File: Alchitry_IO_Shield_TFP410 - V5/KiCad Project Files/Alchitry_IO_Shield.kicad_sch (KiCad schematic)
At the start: 1 part, among them U1 boardmezzanine_new

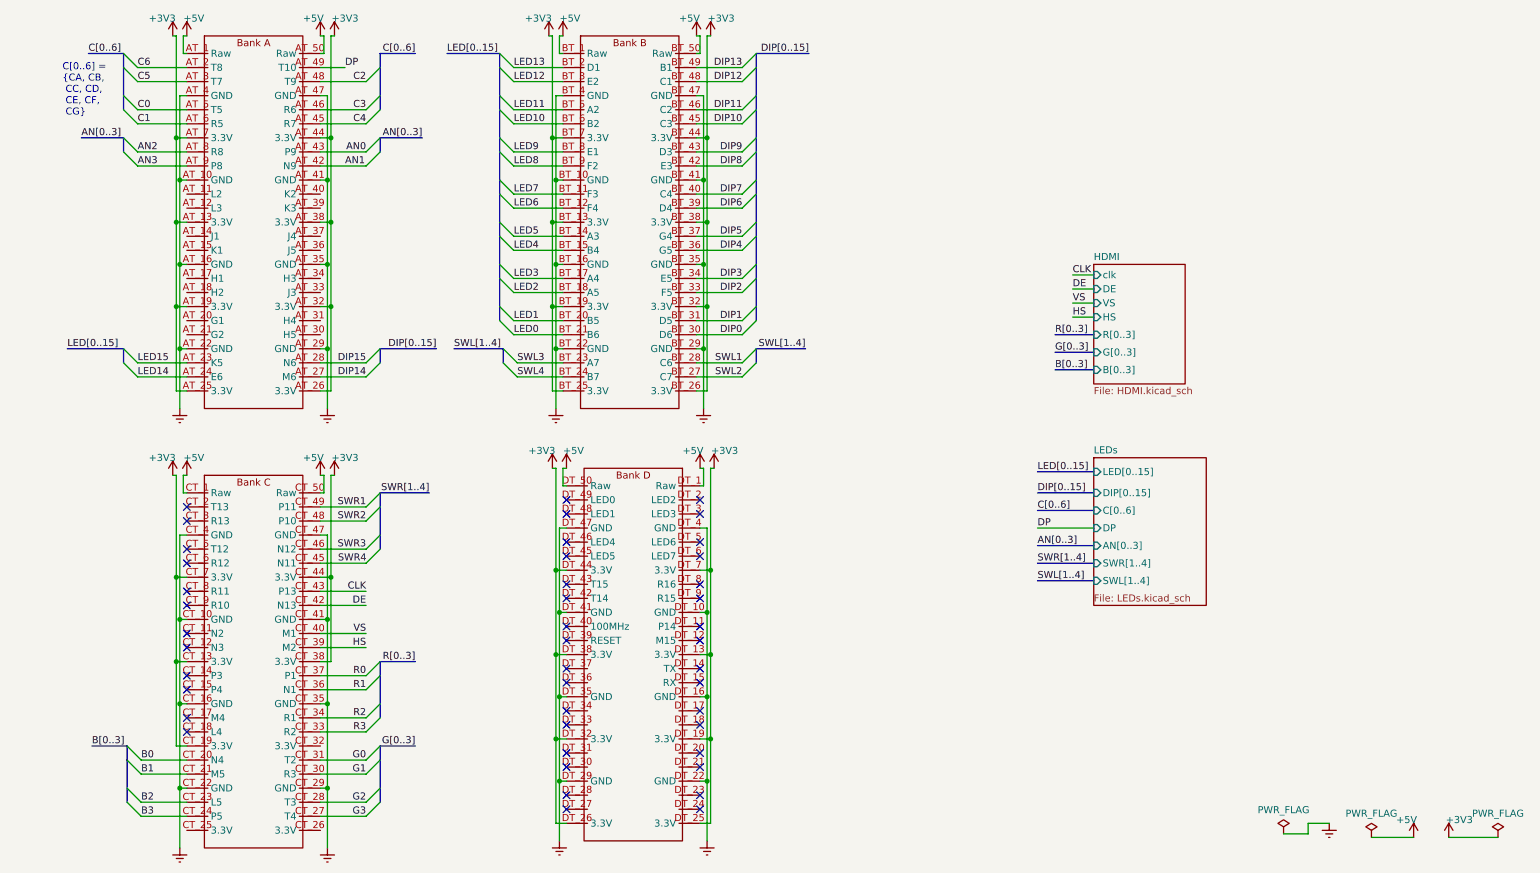
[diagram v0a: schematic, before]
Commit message: started new shield
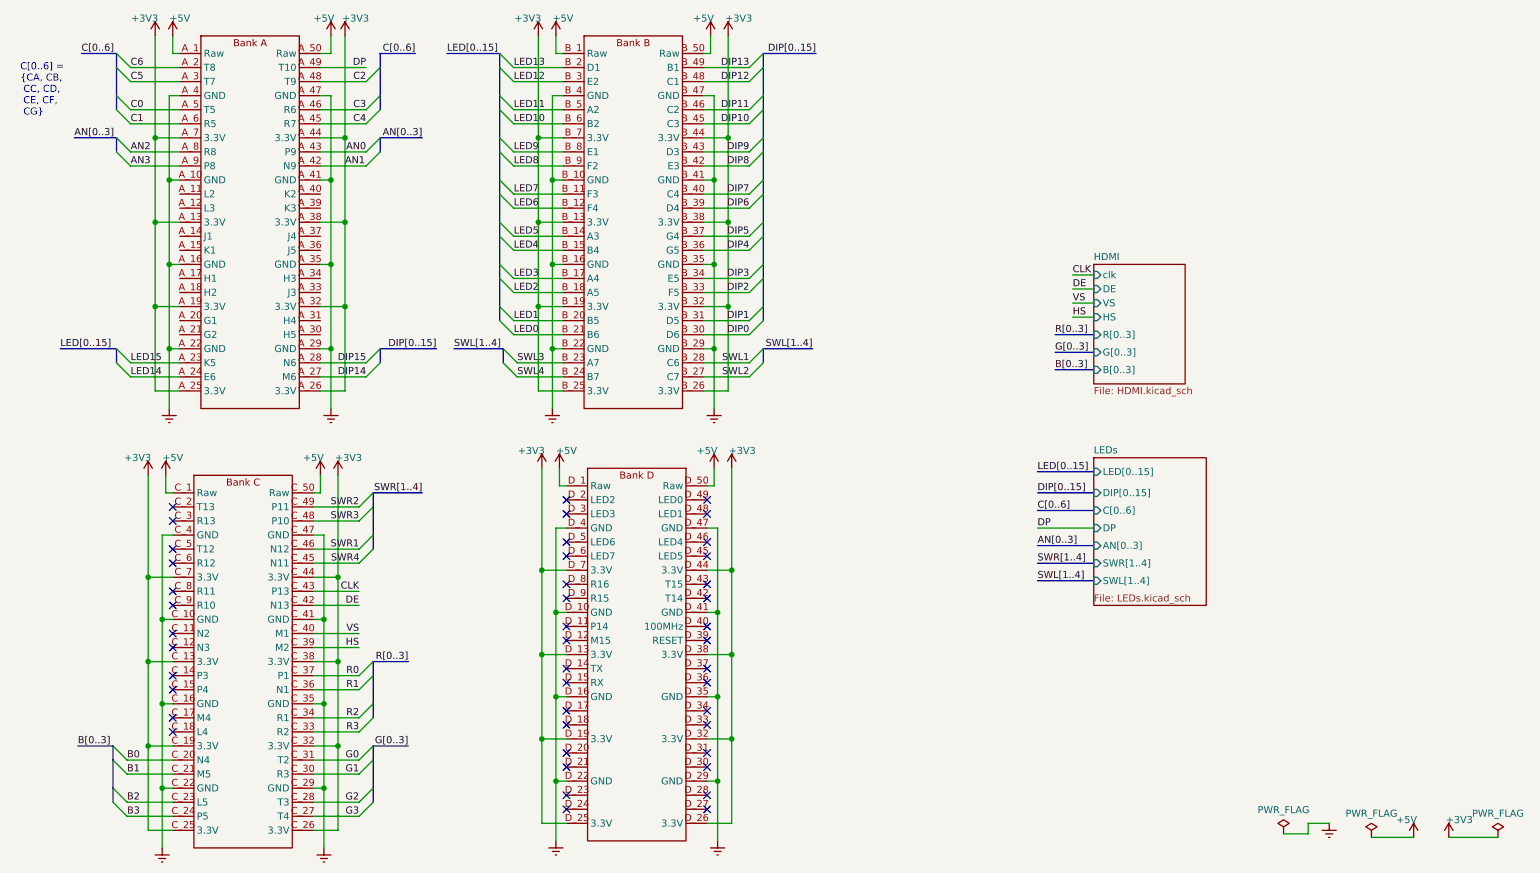
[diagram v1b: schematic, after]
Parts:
- removed U1: boardmezzanine_new, Custom_Parts:Alchitry_Top_Bottom, symbol Custom_Symbols:Adaptor_both-alchitry_symbols
- added U1: Alchitry_Single, Alchitry_Footprints:Alchitry_Bottom, symbol Alchitry_Symbols:Alchitry_Single
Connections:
- net +3V3: now also U1.A_13 (3.3V), U1.A_19 (3.3V), U1.A_25 (3.3V), U1.A_26 (3.3V), U1.A_32 (3.3V), U1.A_38 (3.3V), U1.A_42 (N9), U1.A_44 (3.3V), U1.A_7 (3.3V), U1.B_13 (3.3V), U1.B_19 (3.3V), U1.B_25 (3.3V), U1.B_26 (3.3V), U1.B_32 (3.3V), U1.B_38 (3.3V), U1.B_44 (3.3V), U1.B_7 (3.3V), U1.C_13 (3.3V), U1.C_19 (3.3V), U1.C_25 (3.3V), U1.C_26 (3.3V), U1.C_32 (3.3V), U1.C_38 (3.3V), U1.C_44 (3.3V), U1.C_7 (3.3V), U1.D_13 (3.3V), U1.D_19 (3.3V), U1.D_25 (3.3V), U1.D_26 (3.3V), U1.D_32 (3.3V), U1.D_38 (3.3V), U1.D_44 (3.3V), U1.D_7 (3.3V)
- net +5V: now also U1.A_1 (Raw), U1.A_50 (Raw), U1.B_1 (Raw), U1.B_50 (Raw), U1.C_1 (Raw), U1.C_50 (Raw), U1.D_1 (Raw), U1.D_50 (Raw)
- net AN0: now also U1.A_43 (P9)
- net AN2: now also U1.A_8 (R8)
- net AN3: now also U1.A_9 (P8)
- net B0: now also U1.C_20 (N4)
- net B1: now also U1.C_21 (M5)
- net B2: now also U1.C_23 (L5)
- net B3: now also U1.C_24 (P5)
- net C0: now also U1.A_5 (T5)
- net C1: now also U1.A_6 (R5)
- net C2: now also U1.A_48 (T9)
- net C3: now also U1.A_46 (R6)
- net C4: now also U1.A_45 (R7)
- net C5: now also U1.A_3 (T7)
- net C6: now also U1.A_2 (T8)
- net CLK: now also U1.C_43 (P13)
- net DE: now also U1.C_42 (N13)
- net DIP0: now also U1.B_30 (D6)
- net DIP1: now also U1.B_31 (D5)
- net DIP10: now also U1.B_45 (C3)
- net DIP11: now also U1.B_46 (C2)
- net DIP12: now also U1.B_48 (C1)
- net DIP13: now also U1.B_49 (B1)
- net DIP14: now also U1.A_27 (M6)
- net DIP15: now also U1.A_28 (N6)
- net DIP2: now also U1.B_33 (F5)
- net DIP3: now also U1.B_34 (E5)
- net DIP4: now also U1.B_36 (G5)
- net DIP5: now also U1.B_37 (G4)
- net DIP6: now also U1.B_39 (D4)
- net DIP7: now also U1.B_40 (C4)
- net DIP8: now also U1.B_42 (E3)
- net DIP9: now also U1.B_43 (D3)
- net DP: now also U1.A_49 (T10)
- net G0: now also U1.C_31 (T2)
- net G1: now also U1.C_30 (R3)
- net G2: now also U1.C_28 (T3)
- net G3: now also U1.C_27 (T4)
- net GNDREF: now also U1.A_10 (GND), U1.A_16 (GND), U1.A_22 (GND), U1.A_29 (GND), U1.A_35 (GND), U1.A_4 (GND), U1.A_41 (GND), U1.A_47 (GND), U1.B_10 (GND), U1.B_16 (GND), U1.B_22 (GND), U1.B_29 (GND), U1.B_35 (GND), U1.B_4 (GND), U1.B_41 (GND), U1.B_47 (GND), U1.C_10 (GND), U1.C_16 (GND), U1.C_22 (GND), U1.C_29 (GND), U1.C_35 (GND), U1.C_4 (GND), U1.C_41 (GND), U1.C_47 (GND), U1.D_10 (GND), U1.D_16 (GND), U1.D_22 (GND), U1.D_29 (GND), U1.D_35 (GND), U1.D_4 (GND), U1.D_41 (GND), U1.D_47 (GND)
- net HS: now also U1.C_39 (M2)
- net LED0: now also U1.B_21 (B6)
- net LED1: now also U1.B_20 (B5)
- net LED10: now also U1.B_6 (B2)
- net LED11: now also U1.B_5 (A2)
- net LED12: now also U1.B_3 (E2)
- net LED13: now also U1.B_2 (D1)
- net LED14: now also U1.A_24 (E6)
- net LED15: now also U1.A_23 (K5)
- net LED2: now also U1.B_18 (A5)
- net LED3: now also U1.B_17 (A4)
- net LED4: now also U1.B_15 (B4)
- net LED5: now also U1.B_14 (A3)
- net LED6: now also U1.B_12 (F4)
- net LED7: now also U1.B_11 (F3)
- net LED8: now also U1.B_9 (F2)
- net LED9: now also U1.B_8 (E1)
- net R0: now also U1.C_37 (P1)
- net R1: now also U1.C_36 (N1)
- net R2: now also U1.C_34 (R1)
- net R3: now also U1.C_33 (R2)
- net SWL1: now also U1.B_28 (C6)
- net SWL2: now also U1.B_27 (C7)
- net SWL3: now also U1.B_23 (A7)
- net SWL4: now also U1.B_24 (B7)
- net SWR1: now also U1.C_46 (N12)
- net SWR2: now also U1.C_49 (P11)
- net SWR3: now also U1.C_48 (P10)
- net SWR4: now also U1.C_45 (N11)
- net VS: now also U1.C_40 (M1)
